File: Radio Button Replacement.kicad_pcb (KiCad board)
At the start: 2 copper layers, 40 x 40 mm, 19 parts, among them SW1 SW_Push_SPDT_1_3_2, SW2 SW_Push_SPDT_1_3_2, SW3 SW_Push_SPDT_1_3_2, SW4 SW_Push_SPDT_1_3_2

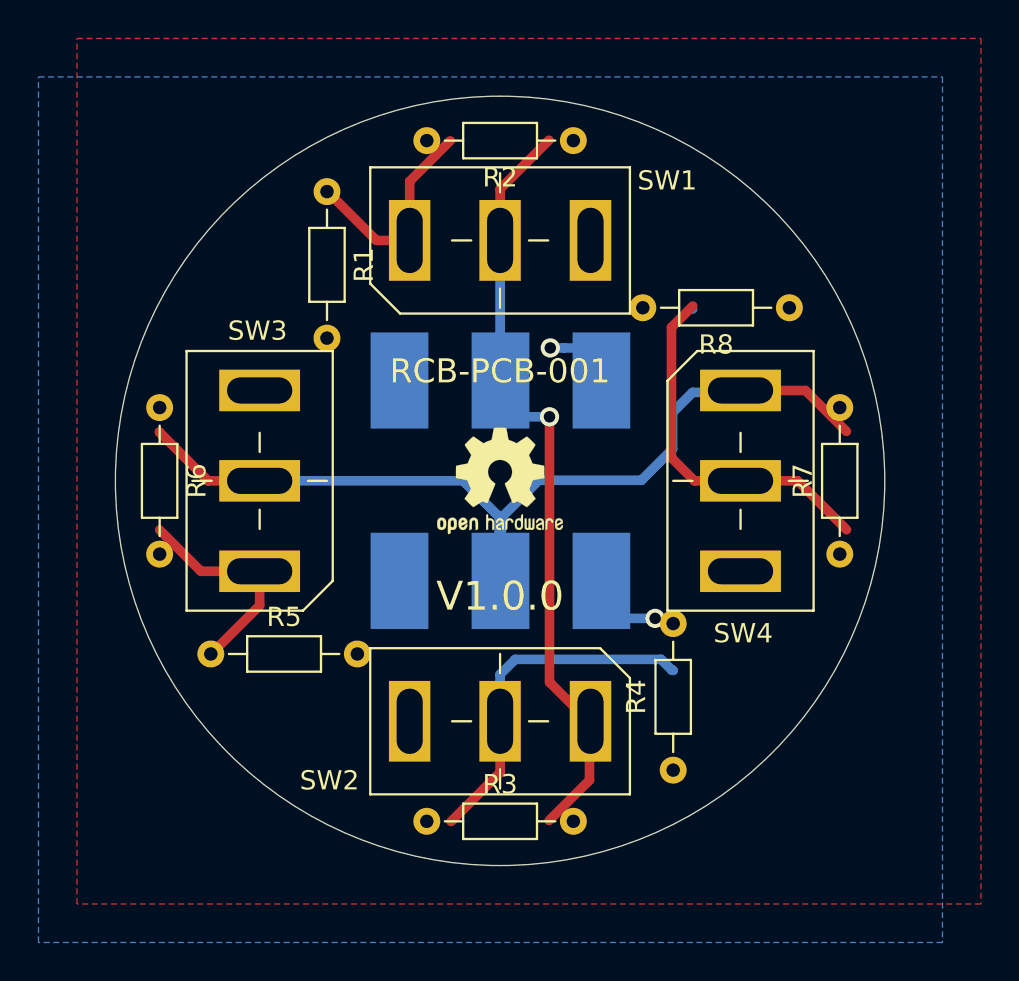
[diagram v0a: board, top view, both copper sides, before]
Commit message: Renumbering of components, PCB updates
Renumbering of components, PCB updates
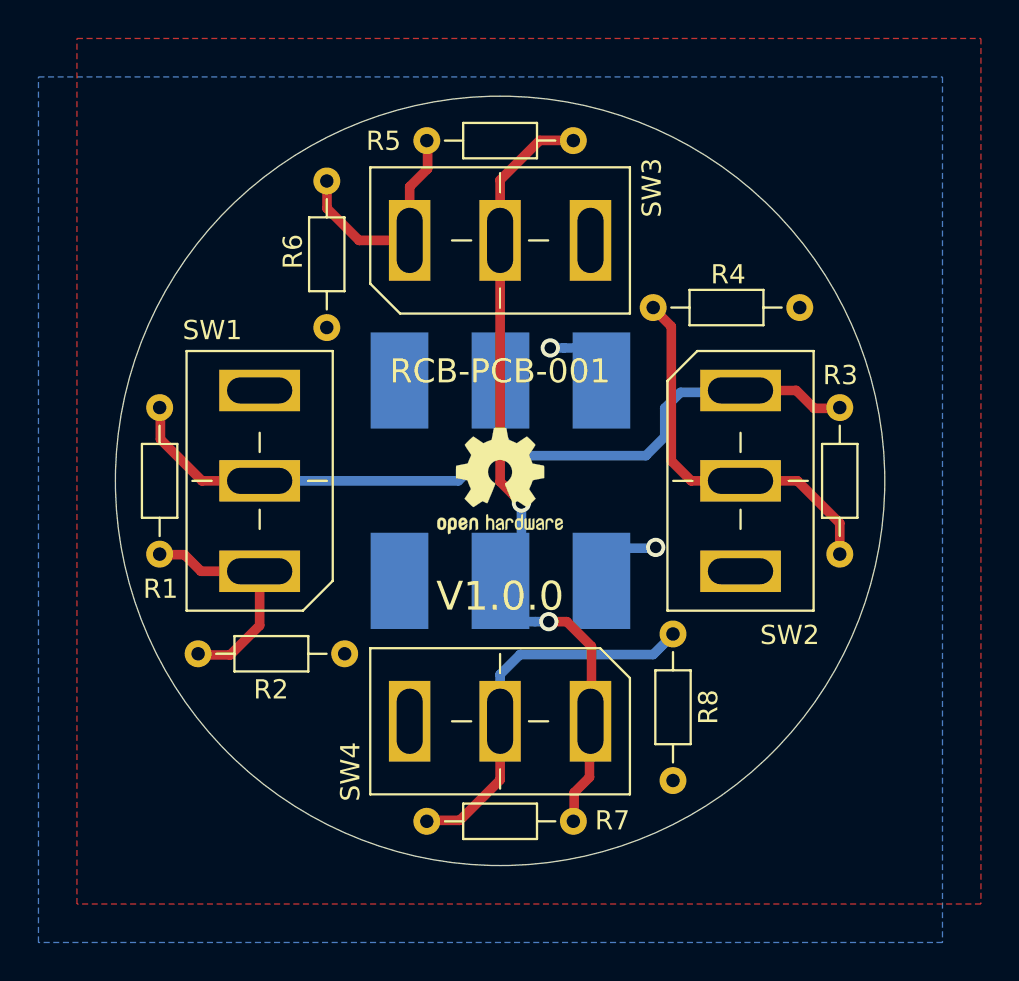
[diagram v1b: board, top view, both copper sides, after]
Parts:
- removed the R8 at (165.0, 91.0)
- added R4: 2.2k, Resistor_THT:R_Axial_DIN0204_L3.6mm_D1.6mm_P7.62mm_Horizontal, F.Cu at (165.6, 91.0)
- moved SW1 17.7 mm to (137.5, 100.0), turned to 180 degrees
- moved SW3 17.7 mm to (150.0, 87.5), turned to 90 degrees
- moved R2 0.66 mm to (134.3, 109.0)
- moved R6 0.55 mm to (141.0, 84.4)
- moved R8 0.54 mm to (159.0, 115.6)
- renumbered R6 to R1, R5 to R2, R7 to R3, R2 to R5, R1 to R6, R3 to R7, R4 to R8, SW4 to SW2, SW2 to SW4
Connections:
- R1 pad 1: /WIRE2 -> /XWIRE
- R1 pad 2: Net-(R5-Pad1) -> Net-(R1-Pad2)
- R2 pad 1: Net-(R5-Pad1) -> Net-(R1-Pad2)
- R3 pad 2: /WIRE2 -> /XWIRE
- R5 pad 1: /WIRE1 -> /YWIRE
- R5 pad 2: Net-(R1-Pad1) -> Net-(R5-Pad2)
- R6 pad 1: Net-(R1-Pad1) -> Net-(R5-Pad2)
- R7 pad 2: /WIRE1 -> /YWIRE
- SW1 pad 1: Net-(R1-Pad1) -> Net-(R1-Pad2)
- SW1 pad 2: /WIRE1 -> /XWIRE
- SW2 pad 1: /WIRE2 -> /XWIRE
- SW3 pad 1: Net-(R5-Pad1) -> Net-(R5-Pad2)
- SW3 pad 2: /WIRE2 -> /YWIRE
- SW4 pad 1: /WIRE1 -> /YWIRE
- TP1 pad 2: /WIRE1 -> /XWIRE
- TP2 pad 2: /WIRE2 -> /YWIRE
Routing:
- net /WIRE2: track 50.2 -> 0.00 mm
- net /XWIRE: track 0.00 -> 47.9 mm
- net /YWIRE: track 0.00 -> 42.9 mm, vias 0 -> 2
- net /WIRE1: track 41.1 -> 0.00 mm, vias 1 -> 0
- net Net-(R1-Pad2): track 0.00 -> 12.1 mm
- net Net-(R5-Pad2): track 0.00 -> 11.9 mm
- net Net-(R1-Pad1): track 11.5 -> 0.00 mm
- net Net-(R5-Pad1): track 11.4 -> 0.00 mm
- net VBUS: track 7.94 -> 5.50 mm
- net Net-(R7-Pad1): track 18.3 -> 20.1 mm
- net Net-(R3-Pad1): track 19.1 -> 20.0 mm
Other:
- board text added: "X"
- board text added: "Y"
- board text removed: "1"
- board text removed: "2"
